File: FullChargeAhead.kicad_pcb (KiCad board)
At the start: 2 copper layers, 38.6 x 25.8 mm, 20 parts, among them P101 CONN_01X02, P102 JST 2 Pin, U101 MCP73834-FCI/UN

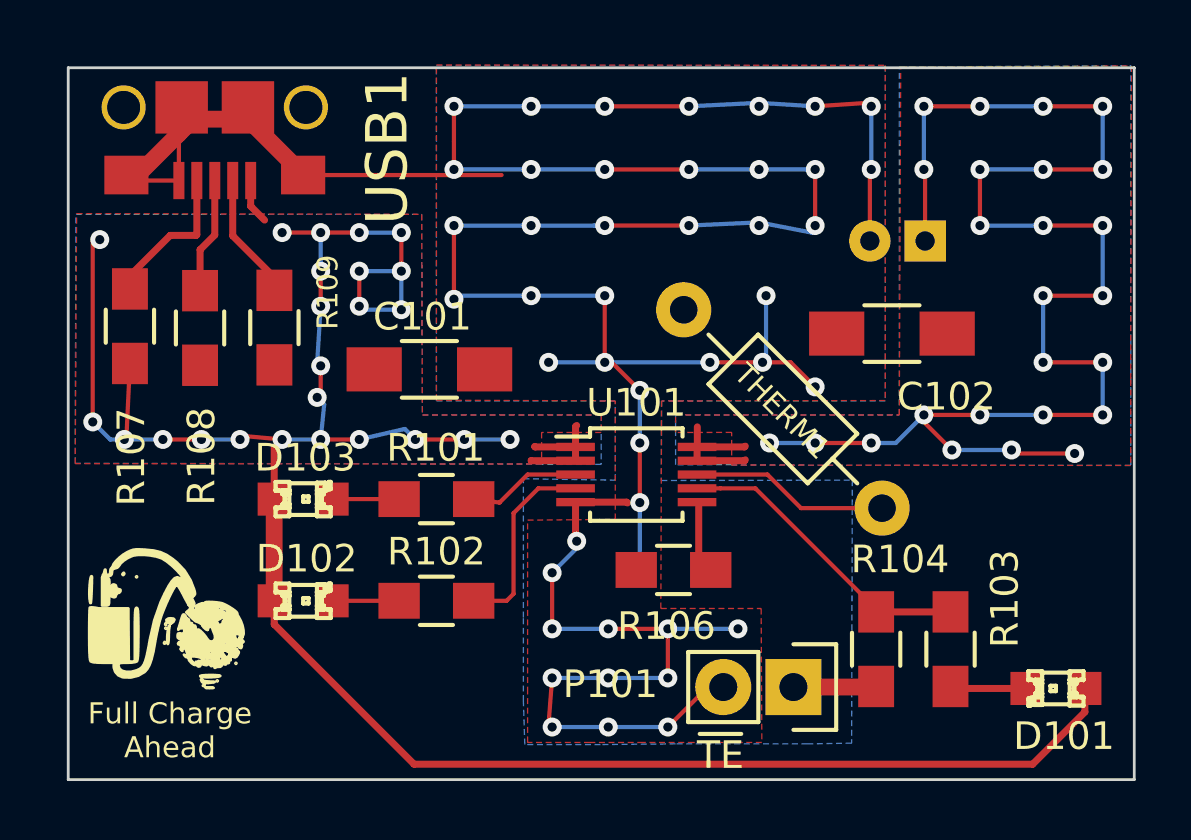
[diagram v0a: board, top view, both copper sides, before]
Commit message: The last final layout and shpark review
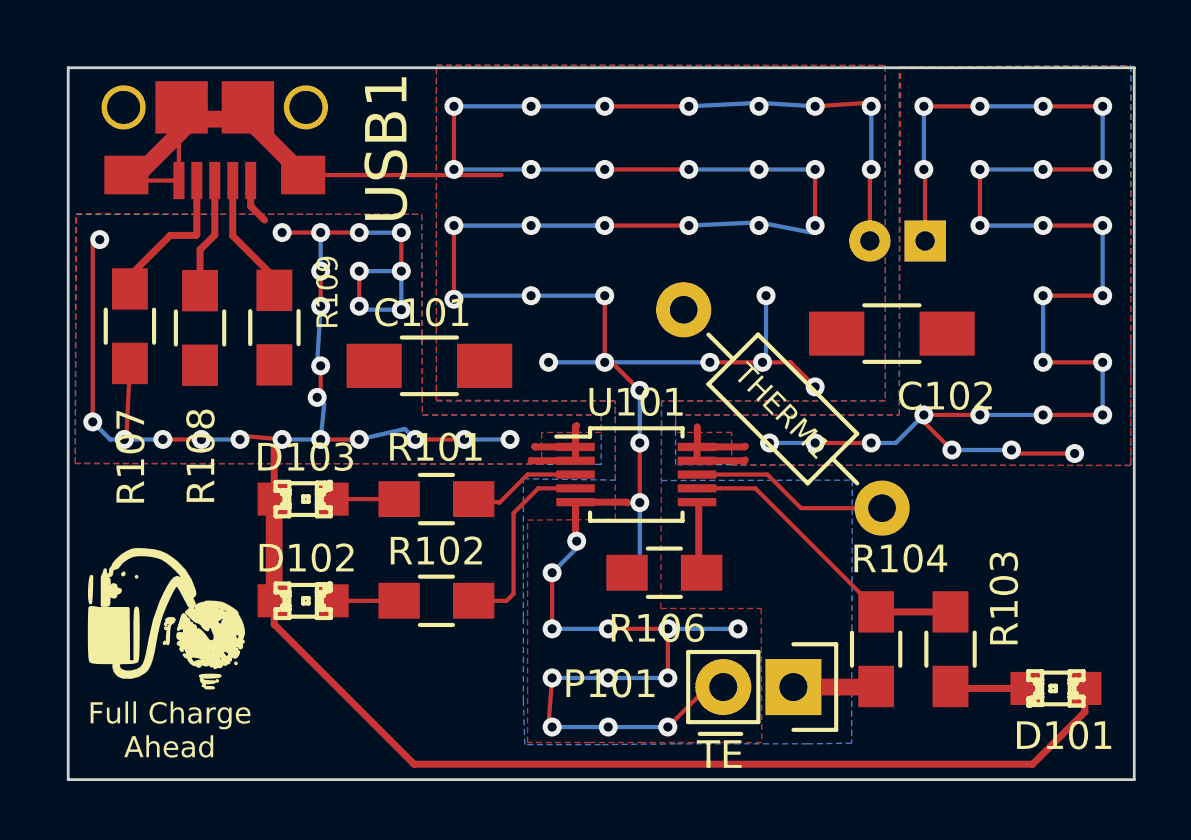
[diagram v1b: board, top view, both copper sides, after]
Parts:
- moved R106 0.35 mm to (108.7, 77.3)
- moved C101 0.13 mm to (100.2, 69.8)
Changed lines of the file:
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@@
     (links 36)
     (no_connects 0)
-    (area 87.071999 59.004999 125.780001 84.886001)
+    (area 83.846057 55.8627 125.780001 84.886001)
     (thickness 1.6)
     (drawings 7)
@@
   )
   (module Capacitors_SMD:C_1206_HandSoldering (layer F.Cu)
-    (at 100.203 69.977)
+    (at 100.203 69.85)
     (descr "Capacitor SMD 1206, hand soldering")
     (tags "capacitor 1206")
@@
   )
   (module Resistors_SMD:R_0805_HandSoldering (layer F.Cu)
-    (at 109.0422 77.2414)
+    (at 108.712 77.343)
     (descr "Resistor SMD 0805, hand soldering")
     (tags "resistor 0805")
